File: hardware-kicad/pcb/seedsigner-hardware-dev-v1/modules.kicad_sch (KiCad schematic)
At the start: 3 parts, among them U1 LuckFox_Pico_MINI, U2 WAVESHARE_LCD_BUTTON_BOARD_1.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, U3 RPI_ZERO

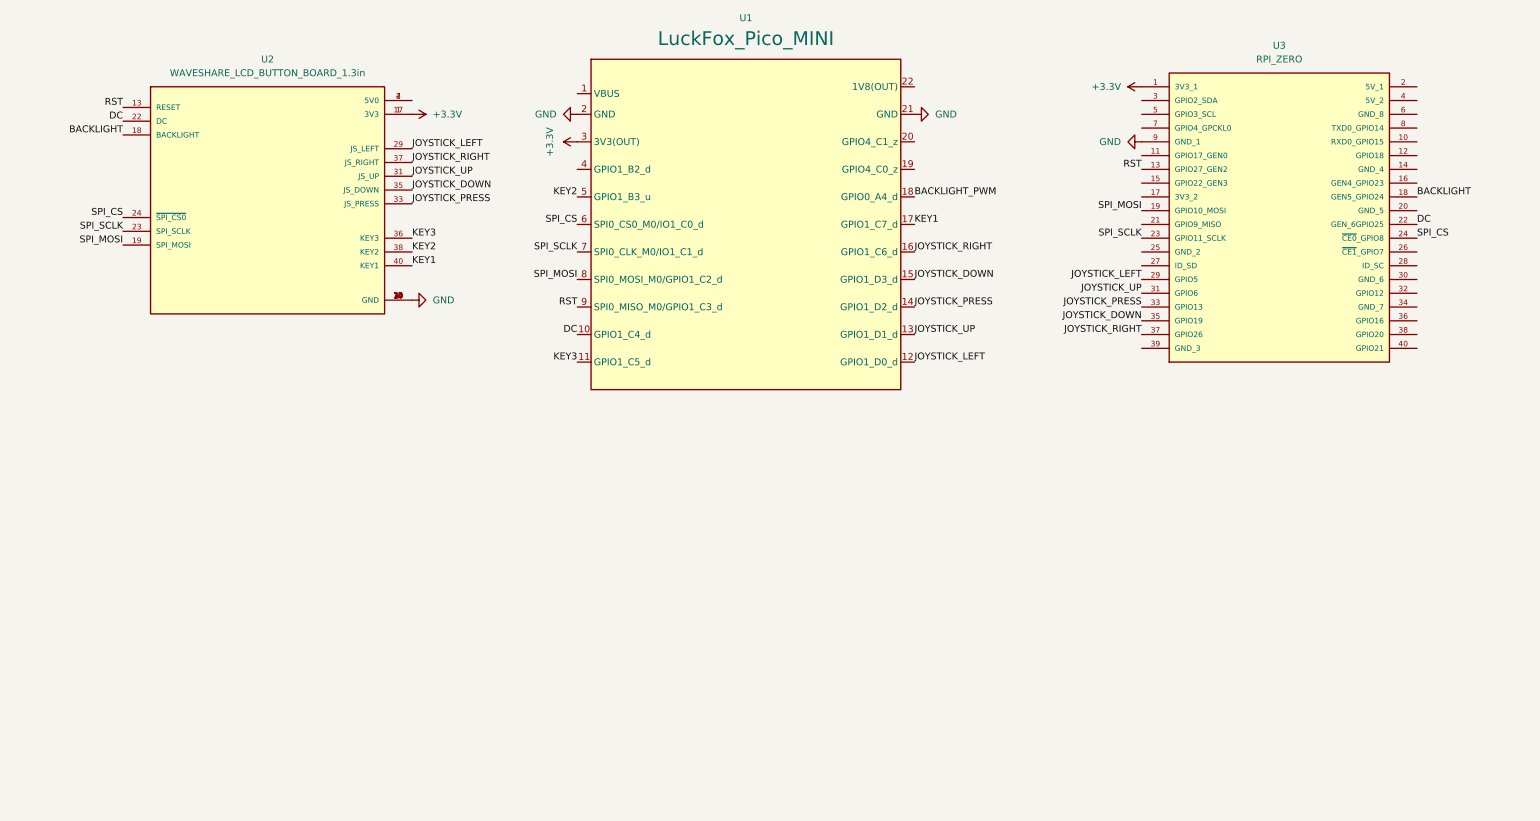
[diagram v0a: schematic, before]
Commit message: 2 different pcbs almost done
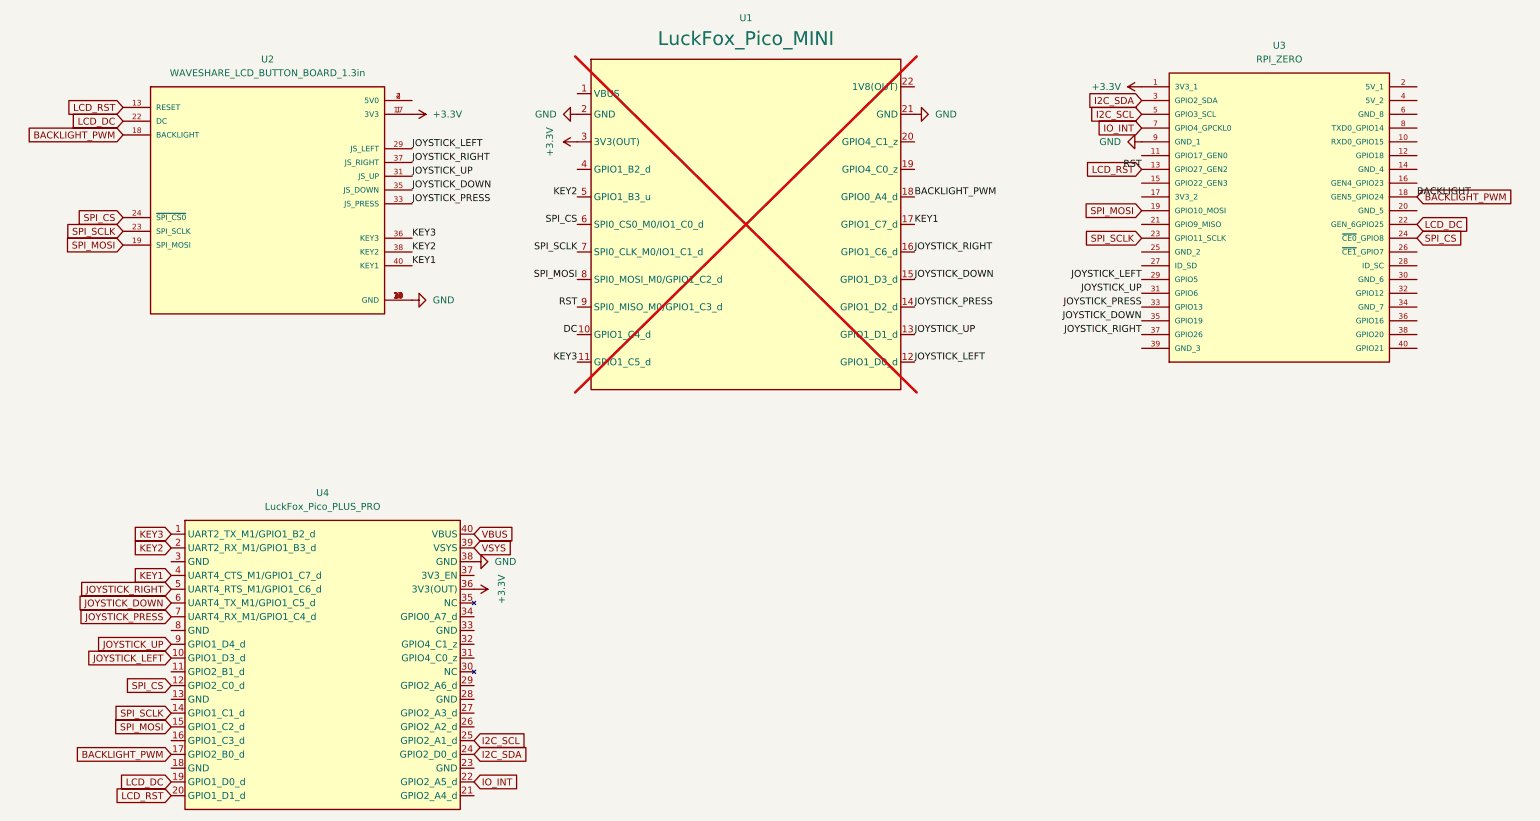
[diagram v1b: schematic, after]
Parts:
- added U4: LuckFox_Pico_PLUS_PRO, seedsigner-luckfox:LUCKFOX_PICO, symbol Luckfox:LuckFox_Pico_PLUS_PRO
- U1: now not fitted; now left out of the parts list
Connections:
- net BACKLIGHT is gone; now on net BACKLIGHT_PWM: U2.18 (BACKLIGHT), U3.18 (GEN5_GPIO24)
- net +3.3V: now also U4.36 (3V3(OUT))
- net BACKLIGHT_PWM: now also U4.17 (GPIO2_B0_d)
- net DC: no longer U2.22 (DC), U3.22 (GEN_6GPIO25)
- net GND: now also U4.38 (GND)
- net JOYSTICK_DOWN: now also U4.6 (UART4_TX_M1/GPIO1_C5_d)
- net JOYSTICK_LEFT: now also U4.10 (GPIO1_D3_d)
- net JOYSTICK_PRESS: now also U4.7 (UART4_RX_M1/GPIO1_C4_d)
- net JOYSTICK_RIGHT: now also U4.5 (UART4_RTS_M1/GPIO1_C6_d)
- net JOYSTICK_UP: now also U4.9 (GPIO1_D4_d)
- net KEY1: now also U4.4 (UART4_CTS_M1/GPIO1_C7_d)
- net KEY2: now also U4.2 (UART2_RX_M1/GPIO1_B3_d)
- net KEY3: now also U4.1 (UART2_TX_M1/GPIO1_B2_d)
- net SPI_CS: now also U4.12 (GPIO2_C0_d)
- net SPI_MOSI: now also U4.15 (GPIO1_C2_d)
- net SPI_SCLK: now also U4.14 (GPIO1_C1_d)
- net I2C_SDA: now reaches U3.3 (GPIO2_SDA)
- net I2C_SDA: now also U4.24 (GPIO2_D0_d)
- net I2C_SCL: now reaches U3.5 (GPIO3_SCL)
- net I2C_SCL: now also U4.25 (GPIO2_A1_d)
- net IO_INT: now reaches U3.7 (GPIO4_GPCKL0)
- net IO_INT: now also U4.22 (GPIO2_A5_d)
- net RST renamed LCD_RST
- net LCD_RST: now also U4.20 (GPIO1_D1_d)
- new net LCD_DC: U2.22 (DC), U3.22 (GEN_6GPIO25), U4.19 (GPIO1_D0_d)
- new net VBUS: U4.40 (VBUS)
- new net VSYS: U4.39 (VSYS)
